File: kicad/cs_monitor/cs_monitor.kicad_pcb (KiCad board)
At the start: 2 copper layers, 60.9 x 44.9 mm, 130 parts, among them J1 Conn_01x01_Female, J2 Conn_01x01_Female, J3 Conn_01x01_Female, J4 Conn, J5 Conn_01x01_Female, J6 Conn_01x01_Female, J7 Conn_01x01_Female, J8 Conn_01x01_Female, J9 Conn_01x01_Female, Q1 5N10, Q2 Q_NMOS_GSD, T1 HY931147C, U1 W5500, U2 OPA354AIDBVR, U3 LM2733XMF, U4 LMR50410XDBVR, U5 NCP1117-3.3, U6 MCP1700x, Y1 25MHz, Y2 16

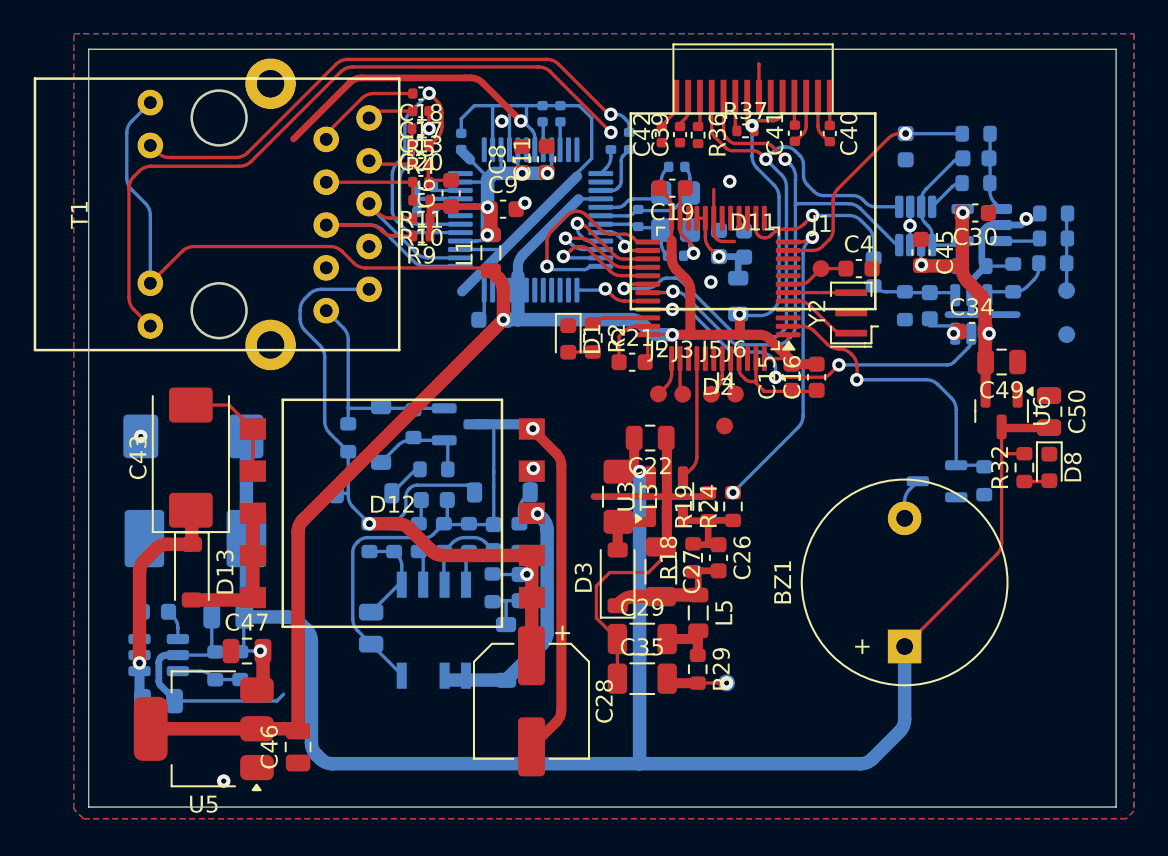
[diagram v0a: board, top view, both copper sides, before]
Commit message: удалено:       kicad/cs_monitor/cs_monitor-backups/cs_monitor-2025-07-08_184829.zip 	удалено:       kicad/cs_monitor/cs_monitor-backups/cs_monitor-2025-07-08_185838.zip 	изменено:      kicad/cs_monitor/cs_monitor.kicad_pcb 	изменено:      kicad/cs_monitor/cs_monitor.kicad_pro 	изменено:      kicad/cs_monitor/cs_monitor.kicad_sch 	изменено:      kicad/cs_monitor/gerber/cs_monitor.drl 	удалено:       kicad/cs_monitor/gerber/cs_monitor_T01_0.30mm.gcode 	удалено:       kicad/cs_monitor/gerber/cs_monitor_T02_0.40mm.gcode 	удалено:       kicad/cs_monitor/gerber/cs_monitor_T03_0.70mm.gcode 	удалено:       kicad/cs_monitor/gerber/cs_monitor_T04_0.76mm.gcode 	удалено:       kicad/cs_monitor/gerber/cs_monitor_T05_1.00mm.gcode 	удалено:       kicad/cs_monitor/gerber/cs_monitor_T06_1.63mm.gcode 	изменено:      stm32cubeide/SC_Monitor/.mxproject 	изменено:      stm32cubeide/SC_Monitor/.settings/language.settings.xml 	изменено:      stm32cubeide/SC_Monitor/Core/Inc/main.h 	изменено:      stm32cubeide/SC_Monitor/Core/Src/main.c 	изменено:      stm32cubeide/SC_Monitor/Release/Core/Src/main.cyclo 	изменено:      stm32cubeide/SC_Monitor/Release/Core/Src/main.o 	изменено:      stm32cubeide/SC_Monitor/Release/Core/Src/main.su 	изменено:      stm32cubeide/SC_Monitor/Release/SC_Monitor.elf 	изменено:      stm32cubeide/SC_Monitor/Release/SC_Monitor.list 	изменено:      stm32cubeide/SC_Monitor/Release/SC_Monitor.map 	изменено:      stm32cubeide/SC_Monitor/SC_Monitor Release.launch 	изменено:      stm32cubeide/SC_Monitor/SC_Monitor.ioc
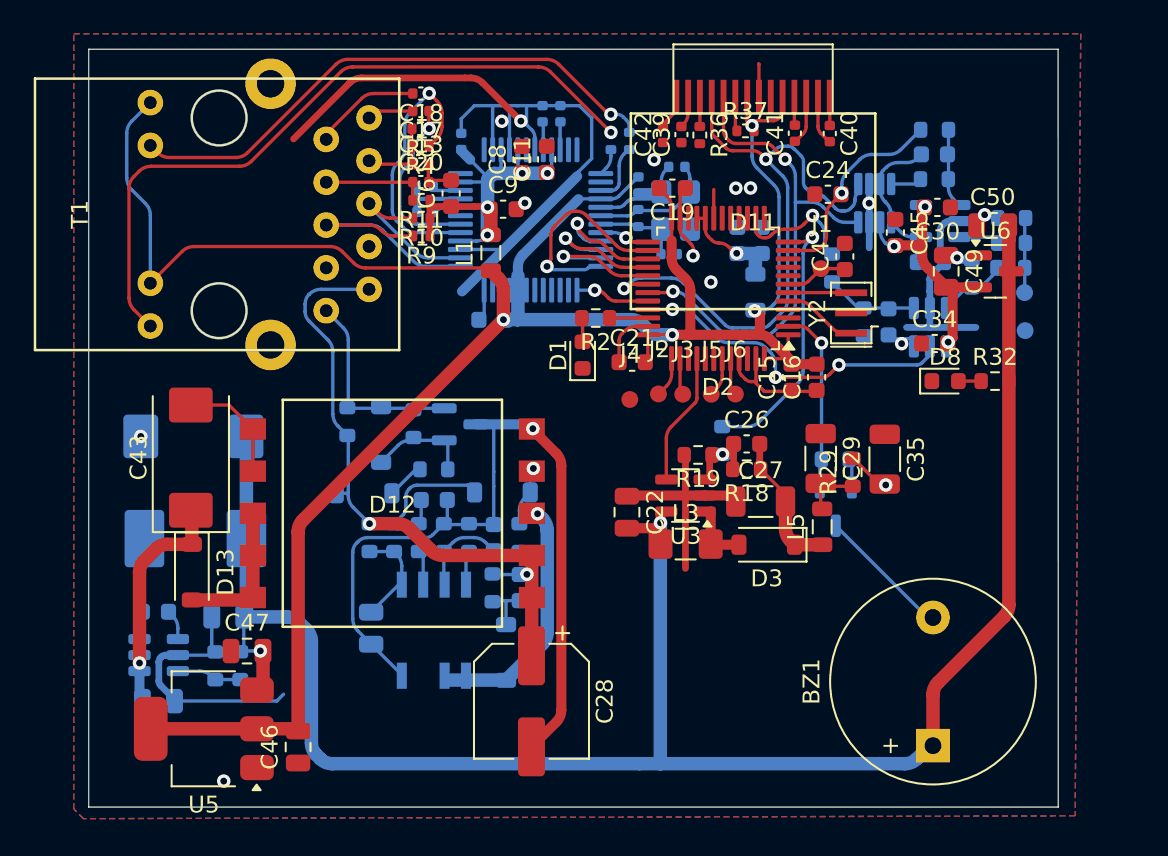
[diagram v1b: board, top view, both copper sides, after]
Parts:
- added C52: 10u, Capacitor_SMD:C_0402_1005Metric, B.Cu at (109.9, 48.8)
- C24: moved to F.Cu
- R24: moved to B.Cu
- moved C35 19.4 mm to (124.5, 65.0), turned to -90 degrees
- moved J8 15.1 mm to (124.5, 66.5)
- moved C29 15.1 mm to (120.7, 65.0), turned to -90 degrees
- moved R29 14.9 mm to (122.6, 65.8), turned to 90 degrees
- moved C50 11.5 mm to (130.9, 51.2), turned to 0 degrees
- moved D3 9.06 mm to (117.5, 70.1), turned to 180 degrees
- moved L5 8.95 mm to (120.8, 69.0), turned to 90 degrees
- moved R39 8.92 mm to (121.6, 65.0), turned to 180 degrees
- moved U6 8.30 mm to (131.1, 53.9), turned to 0 degrees
- moved D8 8.03 mm to (128.1, 60.4), turned to 0 degrees
- moved C27 7.24 mm to (117.1, 67.5), turned to 0 degrees
- moved C26 6.96 mm to (116.3, 64.1), turned to 0 degrees
- moved C49 6.31 mm to (128.1, 53.9), turned to -90 degrees
- moved Q2 6.19 mm to (121.6, 67.8), turned to -90 degrees
- moved R18 6.13 mm to (116.3, 65.6), turned to 180 degrees
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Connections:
- D2 pad 25: INT_ETH -> SS_ETH
- D2 pad 26: SS_ETH -> INT_ETH
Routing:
- net GND: track 152.1 -> 141.6 mm, vias 11 -> 14
- net +5V: track 109.7 -> 116.4 mm
- net Sound: track 17.7 -> 11.1 mm
- net Net-(BZ1-+): track 2.48 -> 8.02 mm
- net SCL: track 34.3 -> 30.0 mm
- net +3V3: track 141.3 -> 144.3 mm
- net Net-(D2-pa6): track 10.2 -> 7.41 mm
- net Pulse: track 22.6 -> 19.9 mm
- net AdjHV: track 18.5 -> 16.0 mm, vias 2 -> 1
- net Analog: track 14.5 -> 12.2 mm
- net SDA: track 39.5 -> 37.6 mm
- net Net-(U3-FB): track 5.84 -> 4.53 mm, vias 0 -> 1
- net +30v: track 3.64 -> 2.53 mm
- net -PoE: track 12.9 -> 12.0 mm
- net Net-(D3-K): track 7.73 -> 8.57 mm
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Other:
- board size 60.9 x 44.9 mm -> 57.5 x 44.9 mm

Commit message: новый файл:    kicad/cs_monitor/bom/ibom.html 	изменено:      kicad/cs_monitor/cs_monitor.kicad_pcb 	изменено:      kicad/cs_monitor/cs_monitor.kicad_sch 	изменено:      stm32cubeide/SC_Monitor/.mxproject 	изменено:      stm32cubeide/SC_Monitor/.settings/language.settings.xml 	изменено:      stm32cubeide/SC_Monitor/Core/Src/main.c 	изменено:      stm32cubeide/SC_Monitor/Release/Core/Src/main.cyclo 	изменено:      stm32cubeide/SC_Monitor/Release/Core/Src/main.o 	изменено:      stm32cubeide/SC_Monitor/Release/Core/Src/main.su 	изменено:      stm32cubeide/SC_Monitor/Release/SC_Monitor.elf 	изменено:      stm32cubeide/SC_Monitor/Release/SC_Monitor.list 	изменено:      stm32cubeide/SC_Monitor/Release/SC_Monitor.map 	изменено:      stm32cubeide/SC_Monitor/SC_Monitor.ioc
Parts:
- C26: value 220p -> 82p
- R18: value 117k -> 120k
- R19: value 5.1k -> 4.3k
- R24: value 50k -> 33k
- R26: value 1.02k -> 1k
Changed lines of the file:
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@@
 			)
 		)
-		(property "Value" "5.1k"
+		(property "Value" "4.3k"
 			(at 0 1.43 0)
 			(layer "F.Fab")
@@
 			)
 		)
-		(property "Value" "117k"
+		(property "Value" "120k"
 			(at 0 1.43 0)
 			(layer "F.Fab")
@@
 			)
 		)
-		(property "Value" "220p"
+		(property "Value" "82p"
 			(at 0 1.43 0)
 			(layer "F.Fab")
@@
 			)
 		)
-		(property "Value" "50k"
+		(property "Value" "33k"
 			(at 0 -1.43 90)
 			(layer "B.Fab")
@@
 			)
 		)
-		(property "Value" "1.02k"
+		(property "Value" "1k"
 			(at 0 -1.43 90)
 			(layer "B.Fab")
